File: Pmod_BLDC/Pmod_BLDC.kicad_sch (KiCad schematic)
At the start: 35 parts, among them IC1 S-5725ECBL0-M3T1U, IC2 S-5725ECBL0-M3T1U, IC3 S-5725ECBL0-M3T1U, J1 Screw_Terminal_01x03, J2 Conn_02x06_Top_Bottom, Q1 TK25S06N1L, Q2 TK25S06N1L, Q3 TK25S06N1L, Q4 TK25S06N1L, Q5 TK25S06N1L, Q6 TK25S06N1L

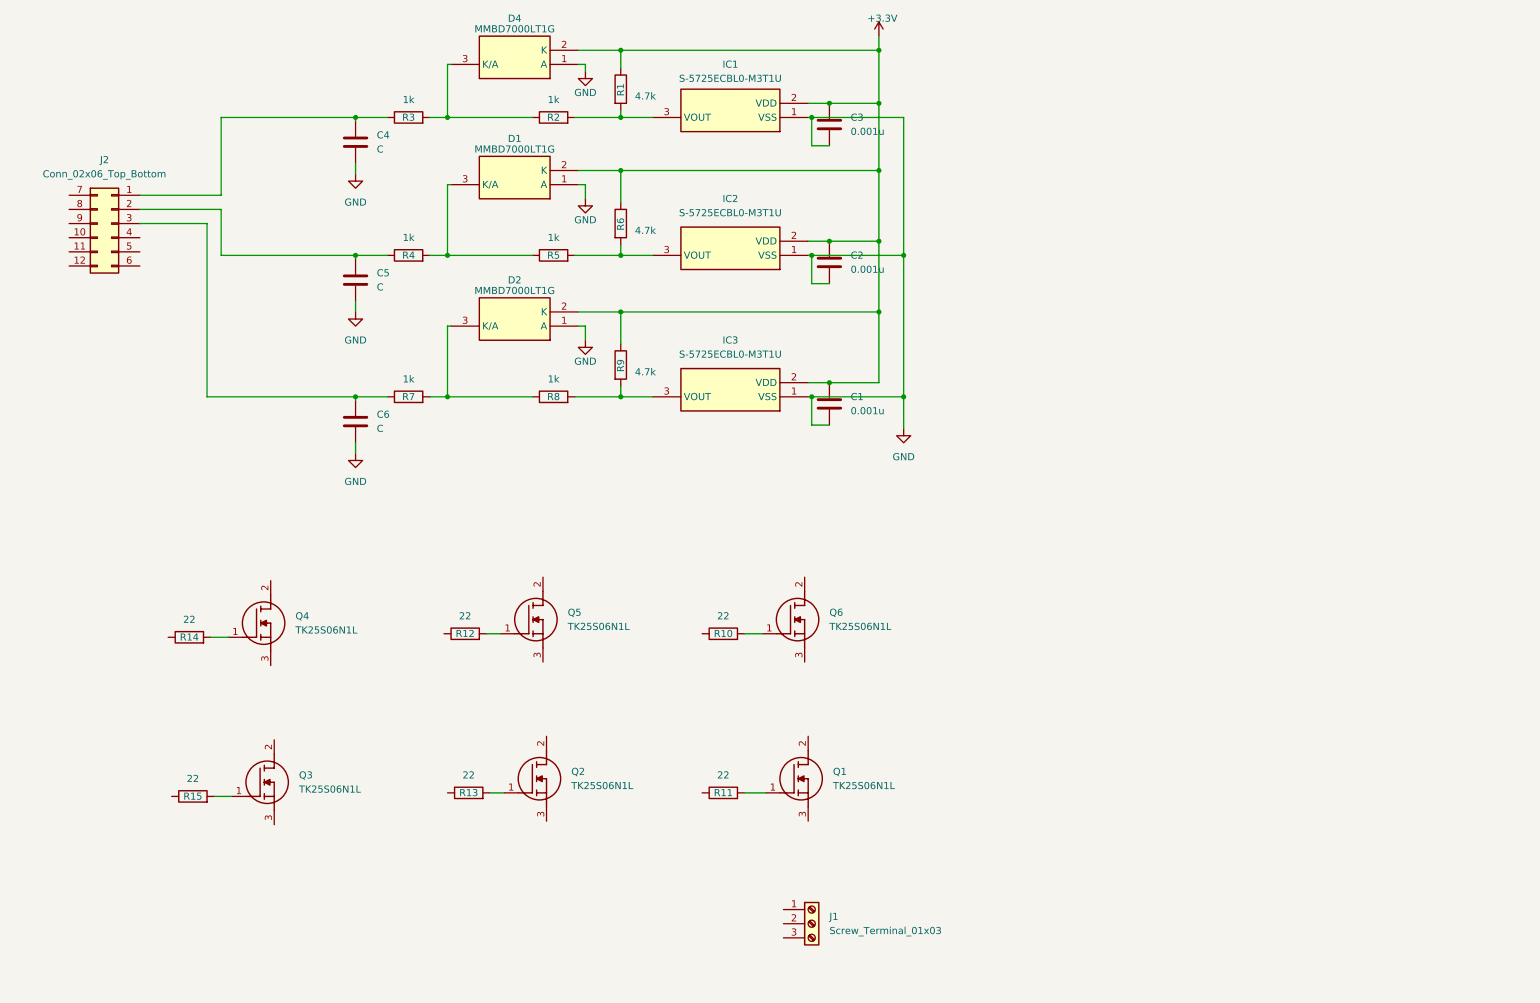
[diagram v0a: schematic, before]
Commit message: 0702
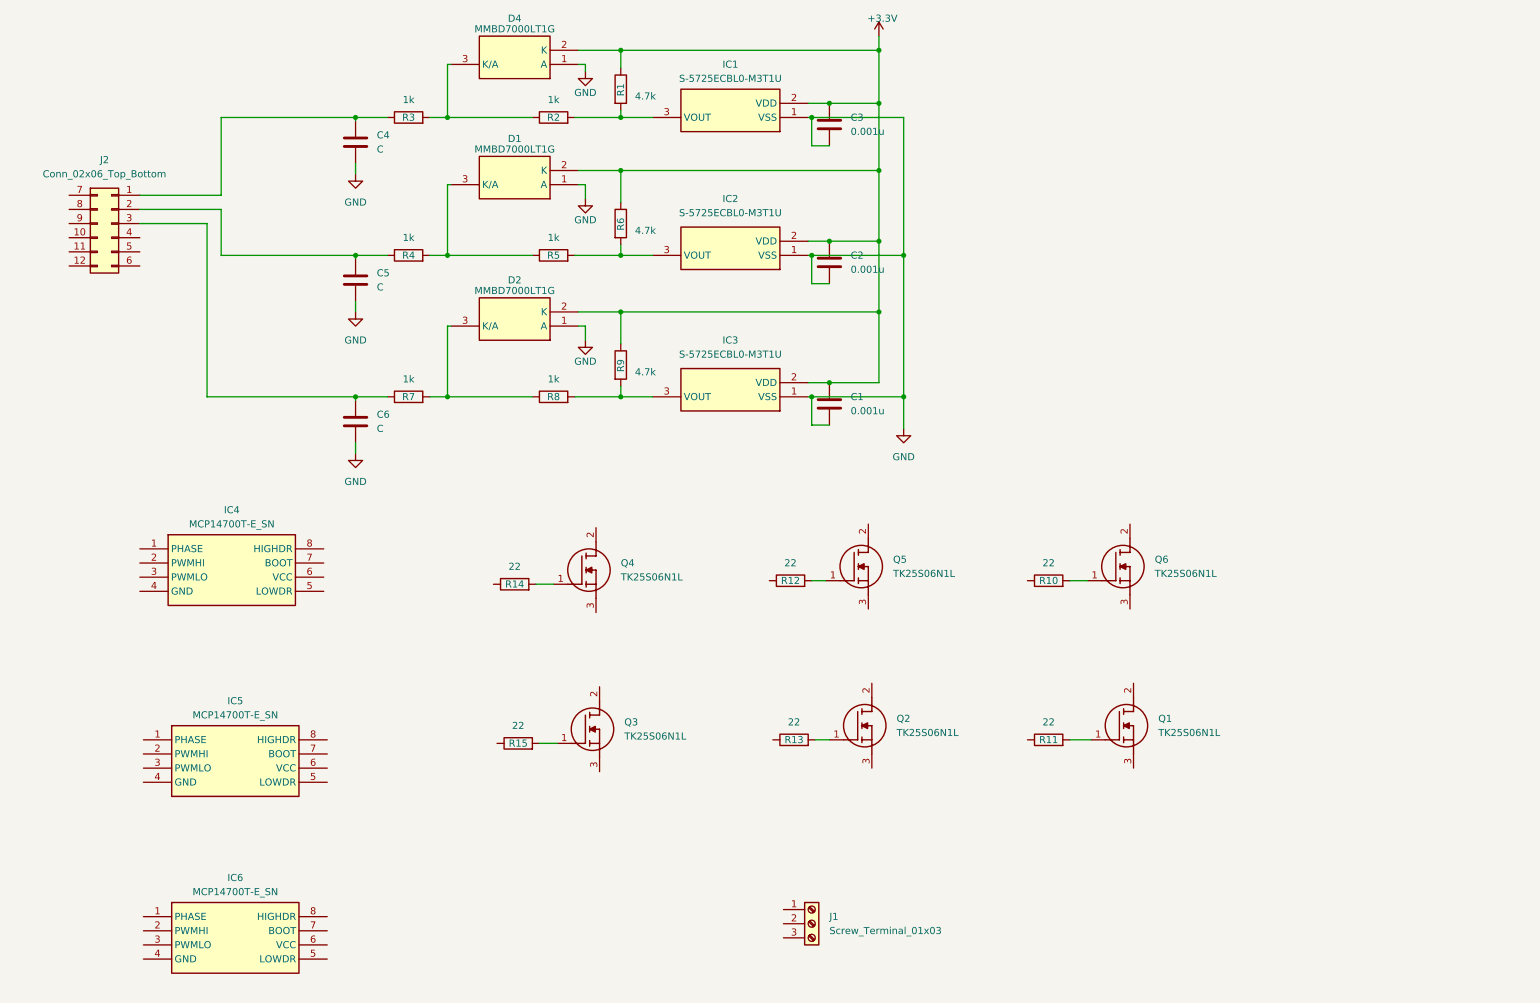
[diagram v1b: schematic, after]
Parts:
- added IC4, IC5, IC6: MCP14700T-E_SN, SOIC127P600X175-8N, symbol samacsys:MCP14700T-E_SN
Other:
- moved on the sheet: Q1, Q2, Q3, Q4, Q5, Q6, R10, R11, R12, R13, R14, R15

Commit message: bldc
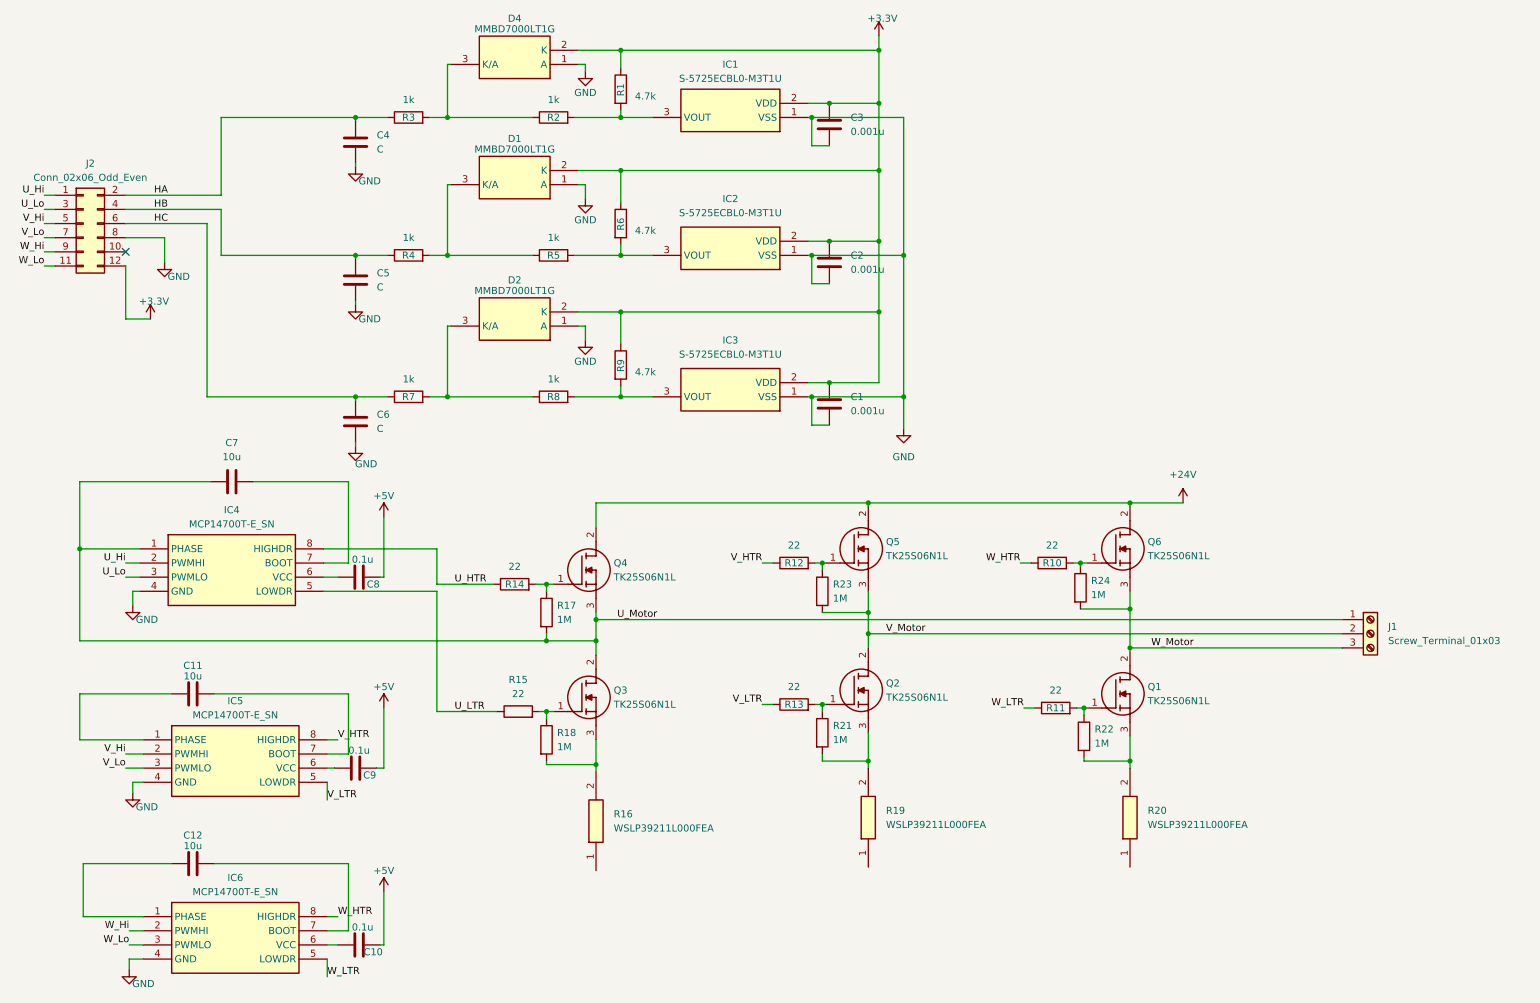
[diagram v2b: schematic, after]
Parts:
- removed J2: Conn_02x06_Top_Bottom, Connector_PinHeader_2.54mm:PinHeader_2x06_P2.54mm_Horizontal, symbol Connector_Generic:Conn_02x06_Top_Bottom
- added C10, C8, C9: 0.1u, Capacitor_SMD:C_0603_1608Metric_Pad1.08x0.95mm_HandSolder, symbol Device:C
- added C11, C12, C7: 10u, Capacitor_SMD:C_1206_3216Metric_Pad1.33x1.80mm_HandSolder, symbol Device:C
- added J2: Conn_02x06_Odd_Even, Connector_PinHeader_2.54mm:PinHeader_2x06_P2.54mm_Vertical, symbol Connector_Generic:Conn_02x06_Odd_Even
- added R16, R19, R20: WSLP39211L000FEA, WSLP39211L000FEA, symbol samacsys:WSLP39211L000FEA
- added R17, R18, R21, R22, R23, R24: 1M, Resistor_SMD:R_0603_1608Metric_Pad0.98x0.95mm_HandSolder, symbol Device:R
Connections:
- net +3.3V: now also J2.12 (Pin_12)
- net GND: now also IC4.4 (GND), IC5.4 (GND), IC6.4 (GND), J2.8 (Pin_8)
- net at Q6.1 (G), R10.2: now also R24.1
- net +24V: now reaches Q6.2 (D)
- net +24V: now also Q4.2 (D), Q5.2 (D)
- net W_Motor: now reaches Q6.3 (S)
- net W_Motor: now also J1.3 (Pin_3), Q1.2 (D), R24.2
- net U_Motor: now reaches J1.1 (Pin_1)
- net U_Motor: now also IC4.1 (PHASE), Q3.2 (D), Q4.3 (S), C7.1, R17.2
- net V_Motor: now reaches J1.2 (Pin_2)
- net V_Motor: now also Q2.2 (D), Q5.3 (S), R23.2
- net V_HTR: now reaches R12.1
- net V_HTR: now also IC5.8 (HIGHDR)
- net at Q5.1 (G), R12.2: now also R23.1
- net HC: now reaches C6.1, R7.1
- net HC: now also J2.6 (Pin_6)
- net at IC6.1 (PHASE): now also C12.1
- net W_Hi: now reaches IC6.2 (PWMHI)
- net W_Hi: now also J2.9 (Pin_9)
- net W_Lo: now reaches IC6.3 (PWMLO)
- net W_Lo: now also J2.11 (Pin_11)
- net W_LTR: now reaches IC6.5 (LOWDR)
- net W_LTR: now also R11.1
- net at IC6.6 (VCC): now also C10.1
- net at IC6.7 (BOOT): now also C12.2
- net W_HTR: now reaches IC6.8 (HIGHDR)
- net W_HTR: now also R10.1
- net HA: now reaches C4.1, R3.1
- net HA: now also J2.2 (Pin_2)
- net HB: now reaches C5.1, R4.1
- net HB: now also J2.4 (Pin_4)
- net at Q1.1 (G), R11.2: now also R22.1
- net U_Hi: now reaches IC4.2 (PWMHI)
- net U_Hi: now also J2.1 (Pin_1)
- net U_Lo: now reaches IC4.3 (PWMLO)
- net U_Lo: now also J2.3 (Pin_3)
- net U_LTR: now reaches IC4.5 (LOWDR)
- net U_LTR: now also R15.1
- net at IC4.6 (VCC): now also C8.1
- net at IC4.7 (BOOT): now also C7.2
- net U_HTR: now reaches IC4.8 (HIGHDR)
- net U_HTR: now also R14.1
- net at Q4.1 (G), R14.2: now also R17.1
- net at Q2.1 (G), R13.2: now also R21.1
- net at Q2.3 (S): now also R19.2, R21.2
- net at Q3.1 (G), R15.2: now also R18.1
- net at IC5.1 (PHASE): now also C11.1
- net V_Hi: now reaches IC5.2 (PWMHI)
- net V_Hi: now also J2.5 (Pin_5)
- net V_Lo: now reaches IC5.3 (PWMLO)
- net V_Lo: now also J2.7 (Pin_7)
- net V_LTR: now reaches IC5.5 (LOWDR)
- net V_LTR: now also R13.1
- net at IC5.6 (VCC): now also C9.1
- net at IC5.7 (BOOT): now also C11.2
- net at Q3.3 (S): now also R16.2, R18.2
- net at Q1.3 (S): now also R20.2, R22.2
- new net +5V: C10.2, C8.2, C9.2
- no-connect marks 0 -> 1
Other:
- moved on the sheet: J1, Q1, Q2, Q3, Q5, Q6, R10, R11, R12, R13, R15
